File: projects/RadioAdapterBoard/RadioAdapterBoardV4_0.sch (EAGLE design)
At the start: 27 parts

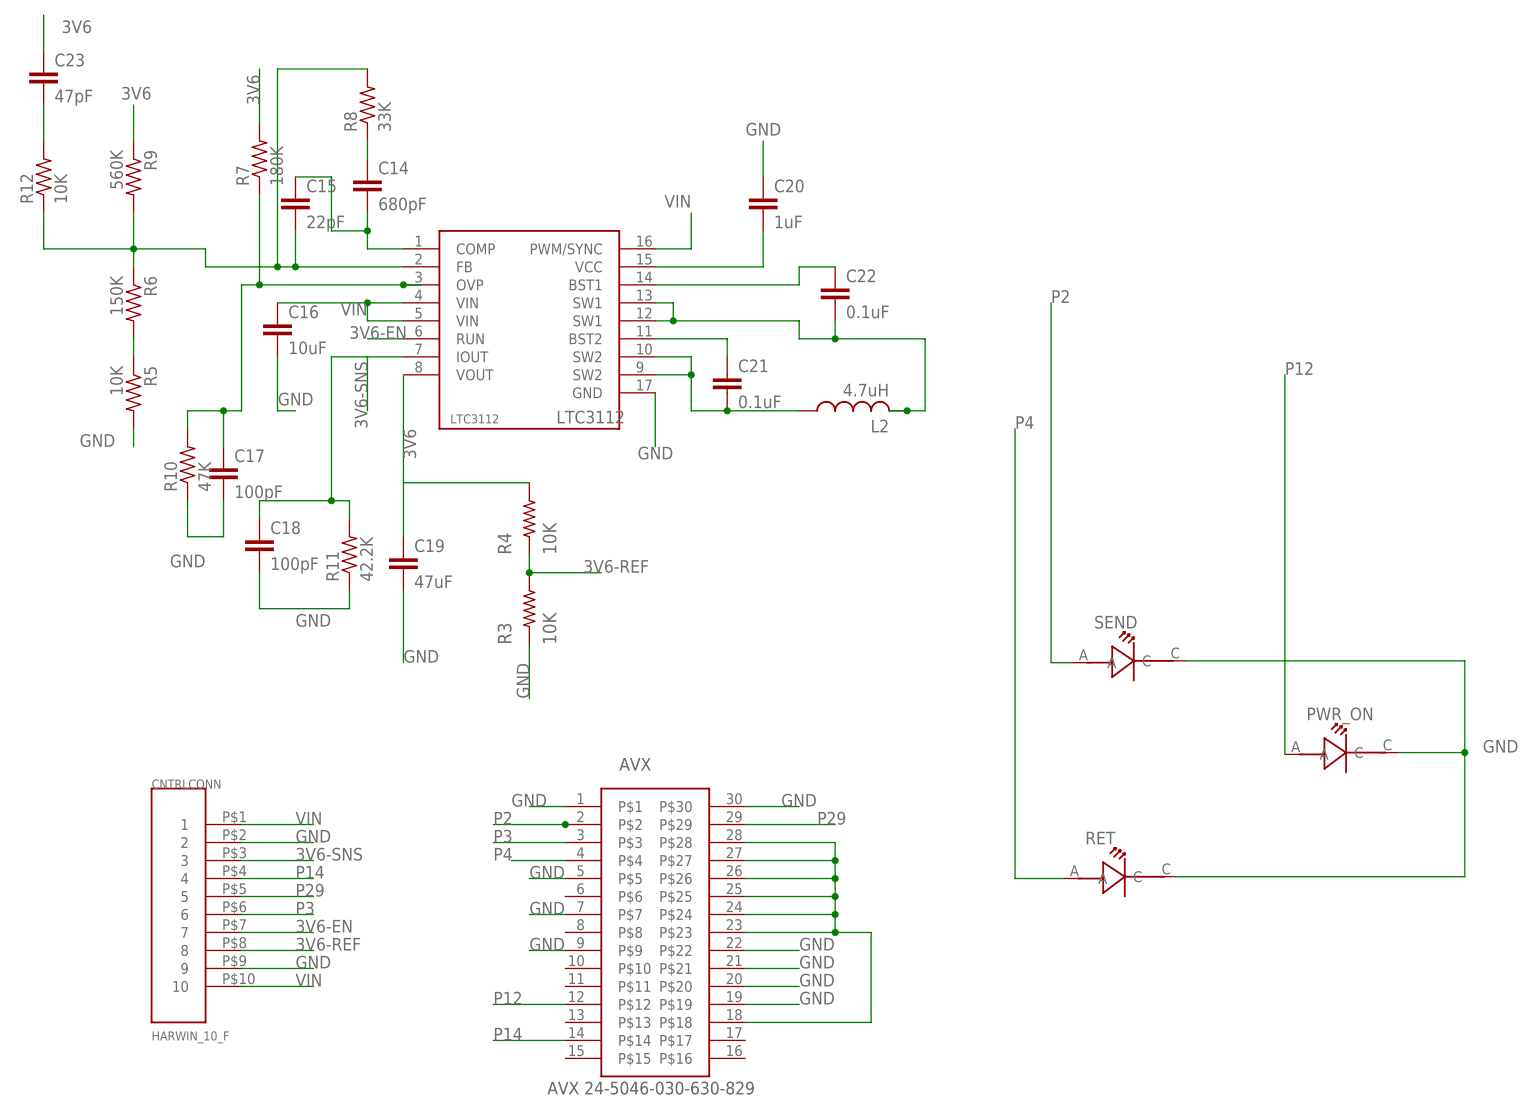
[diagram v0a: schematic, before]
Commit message: Updates to the Radio Adapter Board
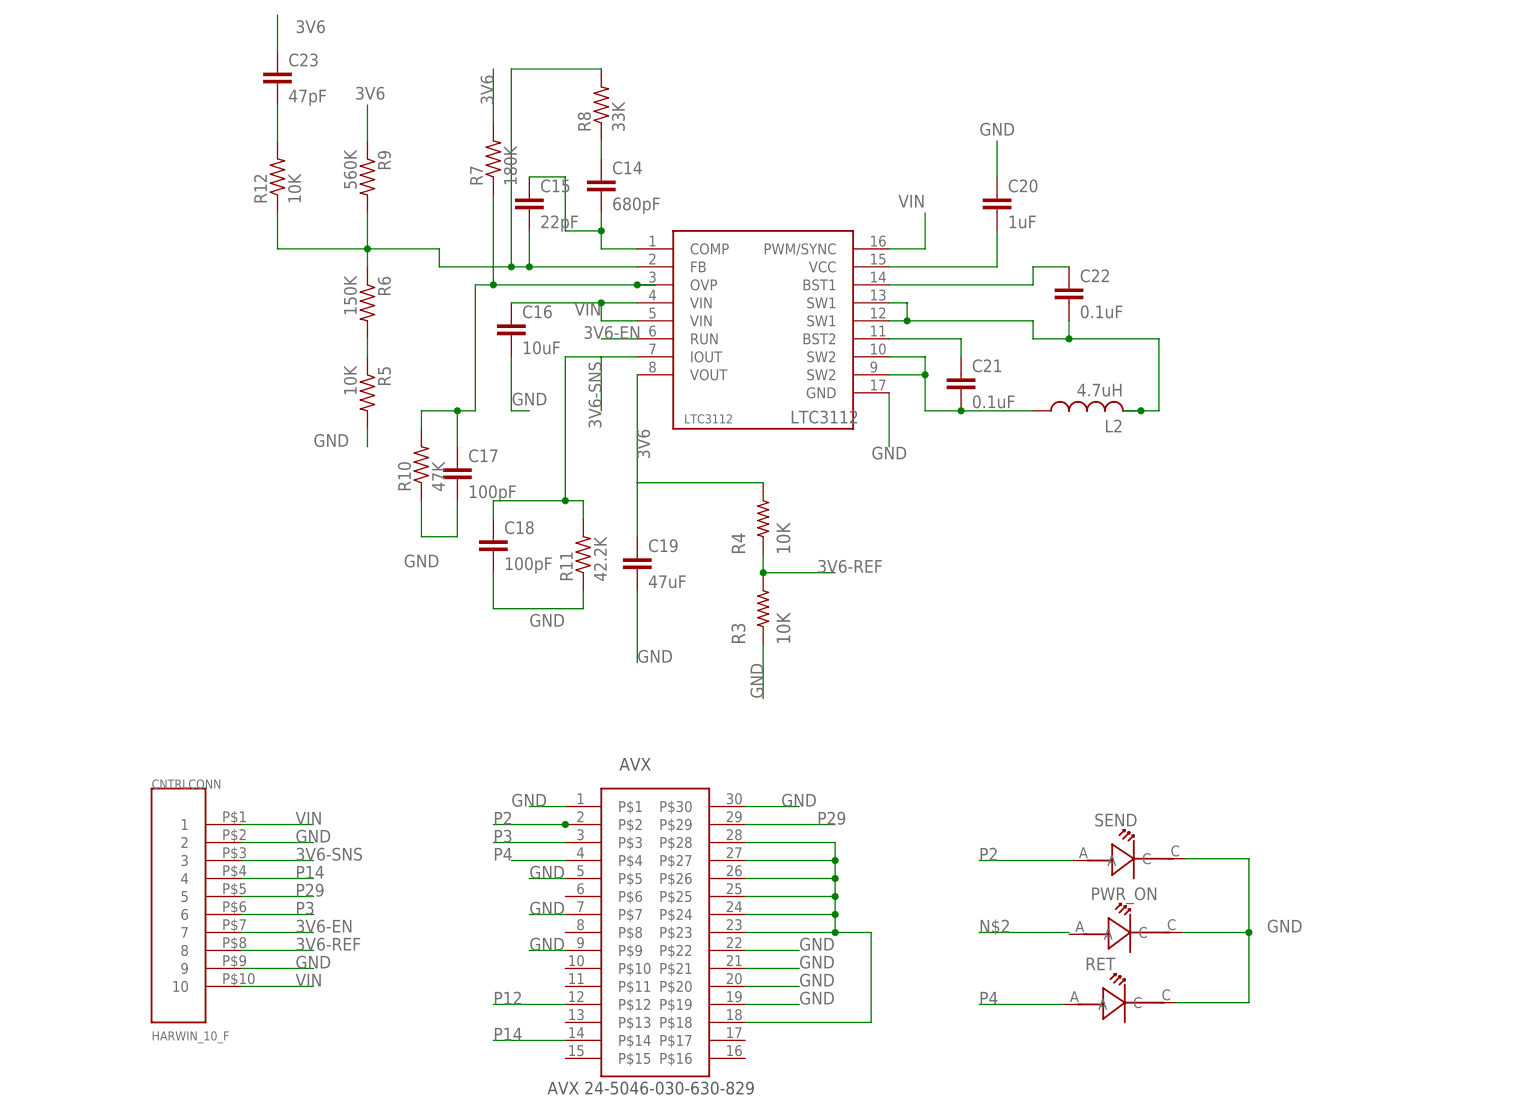
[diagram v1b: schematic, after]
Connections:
- net P12: no longer PWR_ON.A
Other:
- moved on the sheet: C14, C15, C16, C17, C18, C19, C20, C21, C22, C23, L2, LTC3112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
